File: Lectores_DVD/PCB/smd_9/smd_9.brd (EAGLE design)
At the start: 33 x 35.2 mm, 2 parts, among them J1 52793-0970

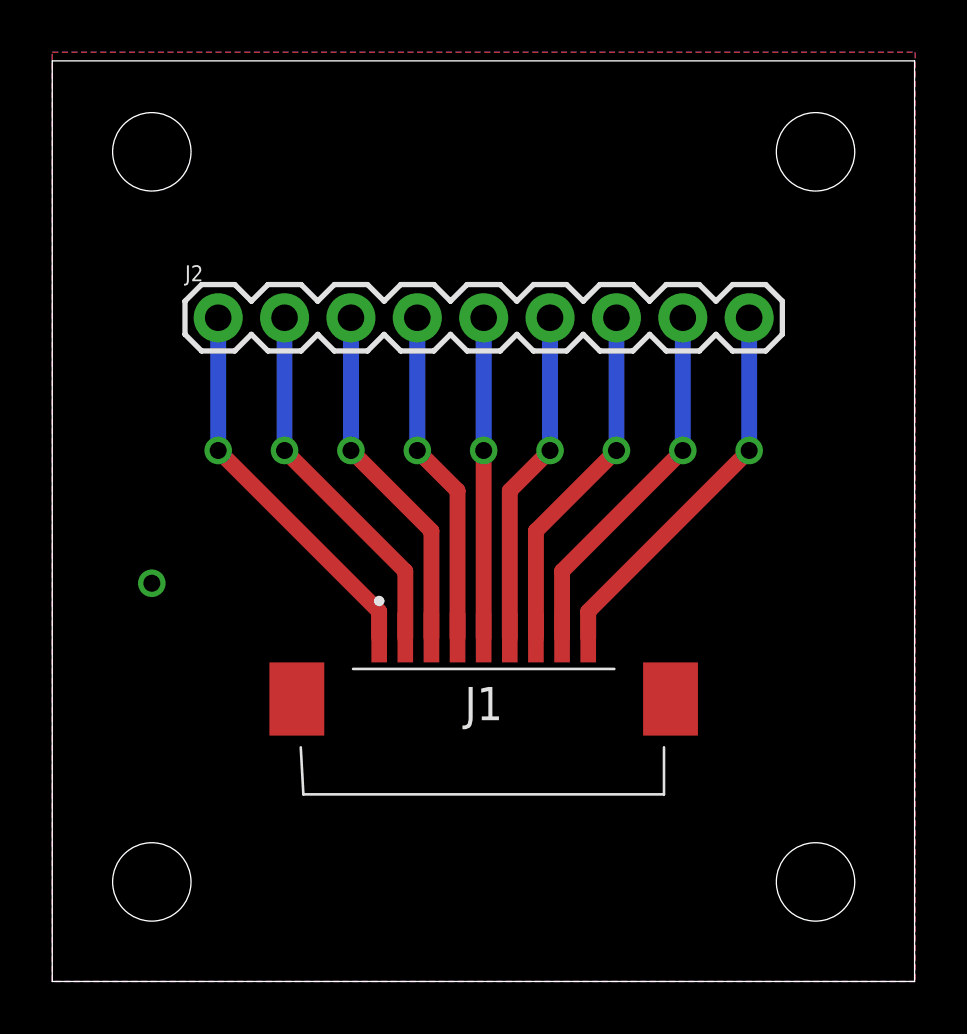
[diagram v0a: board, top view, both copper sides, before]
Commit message: Actualizacion
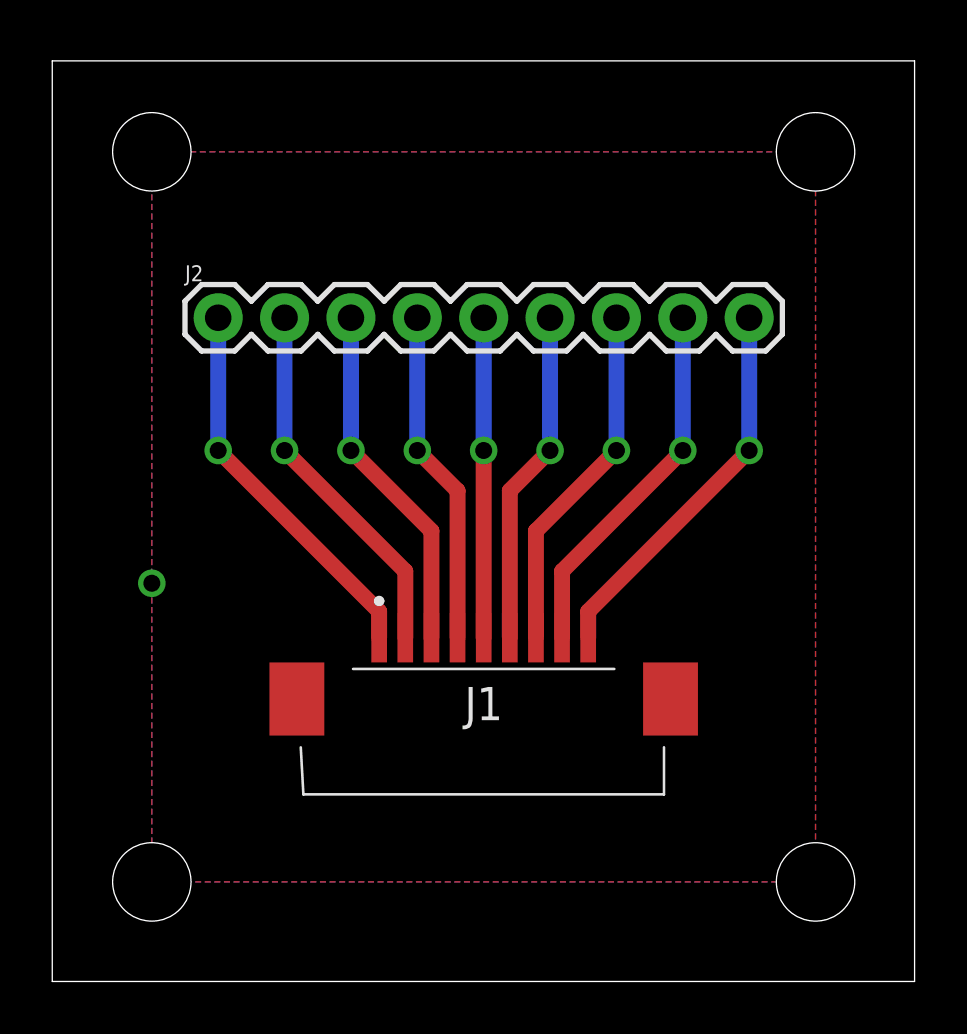
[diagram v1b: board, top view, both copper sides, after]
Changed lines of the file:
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@@
 <signal name="GND">
 <polygon width="0.6096" layer="16">
-<vertex x="0" y="35.56"/>
-<vertex x="33.02" y="35.56"/>
-<vertex x="33.02" y="0"/>
-<vertex x="0" y="0"/>
+<vertex x="3.81" y="31.75"/>
+<vertex x="29.21" y="31.75"/>
+<vertex x="29.21" y="3.81"/>
+<vertex x="3.81" y="3.81"/>
 </polygon>
 <polygon width="0.6096" layer="1">
-<vertex x="0" y="35.56"/>
-<vertex x="33.02" y="35.56"/>
-<vertex x="33.02" y="0"/>
-<vertex x="0" y="0"/>
+<vertex x="3.81" y="31.75"/>
+<vertex x="29.21" y="31.75"/>
+<vertex x="29.21" y="3.81"/>
+<vertex x="3.81" y="3.81"/>
 </polygon>
 <via x="3.81" y="15.24" extent="1-16" drill="0.65"/>
